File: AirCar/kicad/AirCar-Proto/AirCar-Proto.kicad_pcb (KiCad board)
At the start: 2 copper layers, 1 part, among them U1 Pico

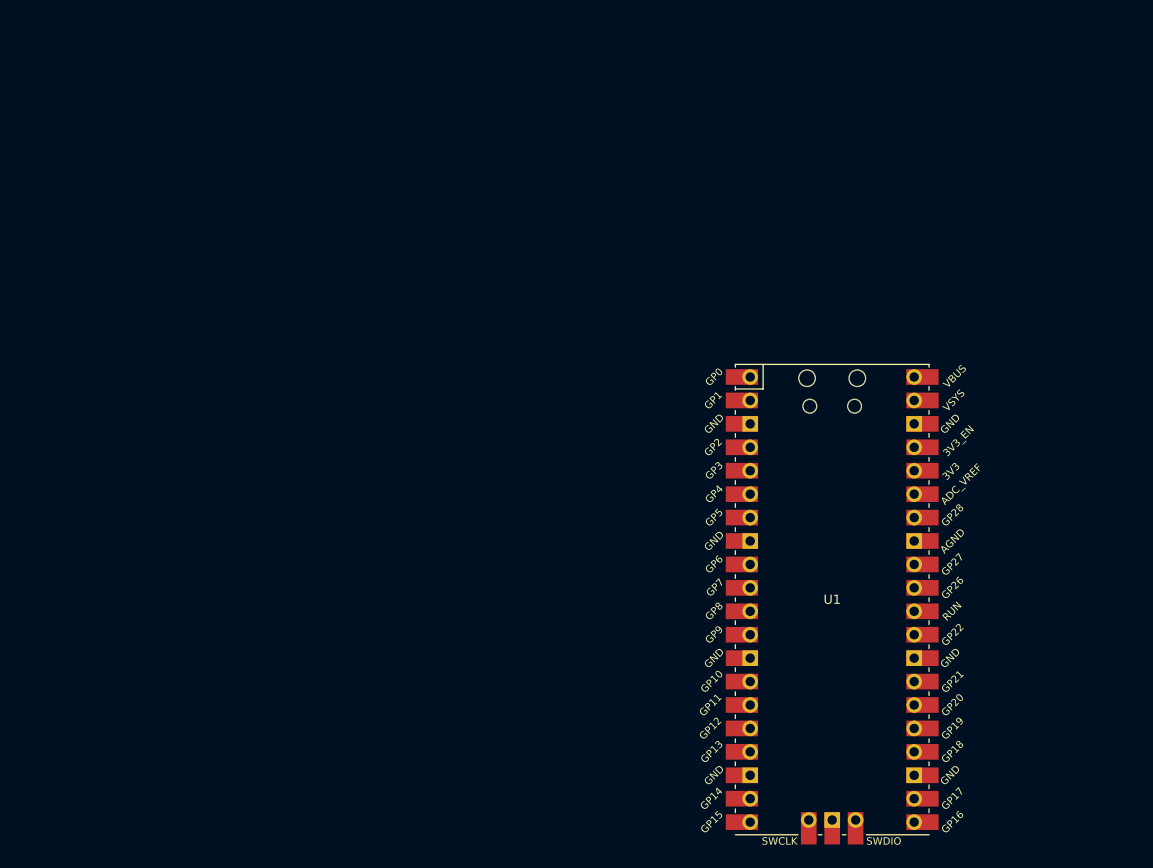
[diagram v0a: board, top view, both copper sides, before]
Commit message: work on proto
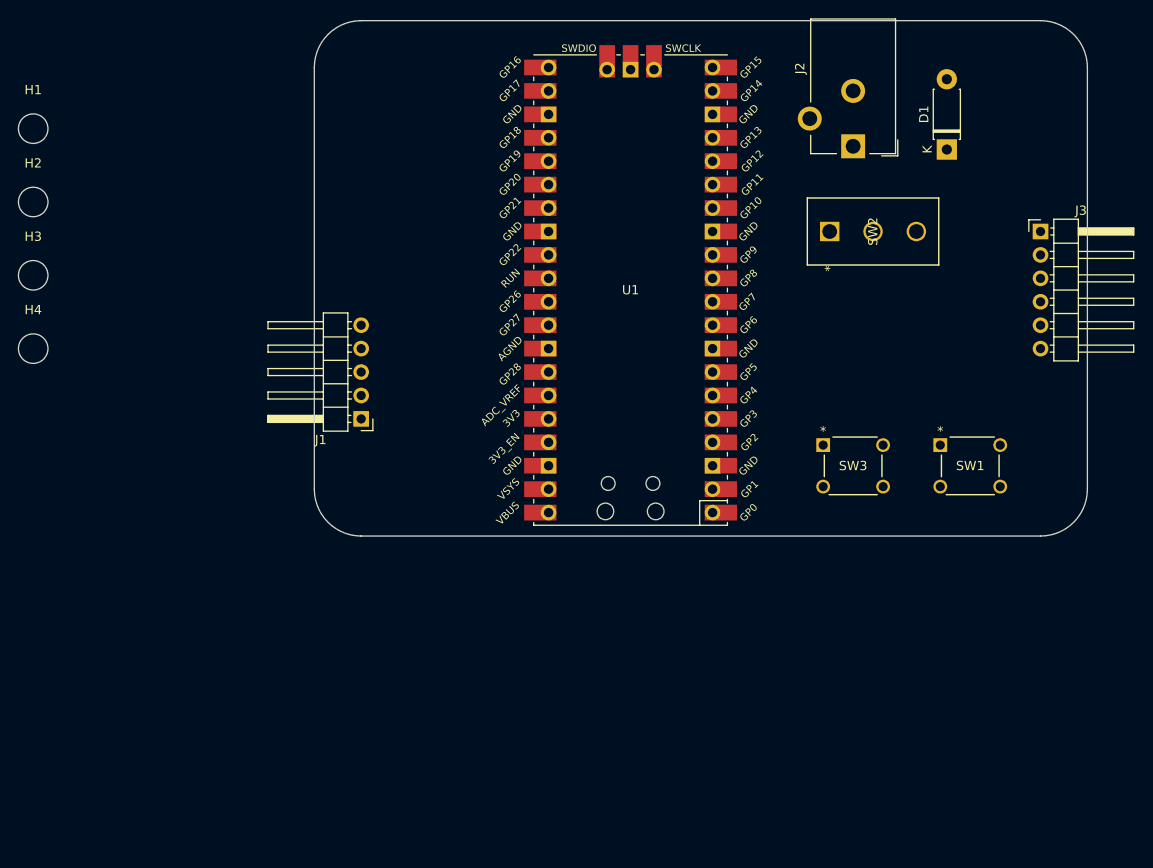
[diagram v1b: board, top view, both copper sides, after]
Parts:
- added D1: D_Schottky, Diode_THT:D_DO-41_SOD81_P7.62mm_Horizontal, F.Cu at (167.6, 39.4)
- added H1: MountingHole, MountingHole:MountingHole_3.2mm_M3, F.Cu at (68.6, 37.1)
- added H2: MountingHole, MountingHole:MountingHole_3.2mm_M3, F.Cu at (68.6, 45.1)
- added H3: MountingHole, MountingHole:MountingHole_3.2mm_M3, F.Cu at (68.6, 53.0)
- added H4: MountingHole, MountingHole:MountingHole_3.2mm_M3, F.Cu at (68.6, 61.0)
- added J1: Conn_01x05, Connector_PinHeader_2.54mm:PinHeader_1x05_P2.54mm_Horizontal, F.Cu at (104.1, 68.6)
- added J2: Barrel_Jack, Connector_BarrelJack:BarrelJack_CUI_PJ-102AH_Horizontal, F.Cu at (157.5, 39.0)
- added J3: Conn_01x06, Connector_PinHeader_2.54mm:PinHeader_1x06_P2.54mm_Horizontal, F.Cu at (177.8, 48.3)
- added SW1: SW_Push, Library:SW4_1825910-B_TEC, F.Cu at (173.4, 75.9)
- added SW2: SW_SPDT, Library:CS12ANW03_NKK, F.Cu at (154.9, 48.3)
- added SW3: SW_Push, Library:SW4_1825910-B_TEC, F.Cu at (160.7, 75.9)
- moved U1 40.1 mm to (133.3, 54.6), turned to 180 degrees
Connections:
- U1 pad 18: unconnected-(U1-GND-Pad18) -> GND
- U1 pad 23: Net-(J1-Pin_1) -> GND
- U1 pad 28: unconnected-(U1-GND-Pad28) -> GND
- U1 pad 3: unconnected-(U1-GND-Pad3) -> GND
- U1 pad 33: unconnected-(U1-AGND-Pad33) -> GND
- U1 pad 39: Net-(D1-K) -> /VSYS
- U1 pad 42: Net-(J3-Pin_2) -> GND
- U1 pad 8: unconnected-(U1-GND-Pad8) -> GND
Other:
- board outline added: 83.8 x 55.9 mm
